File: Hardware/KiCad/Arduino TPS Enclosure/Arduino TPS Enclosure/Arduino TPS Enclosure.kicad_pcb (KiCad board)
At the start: 2 copper layers, 73.7 x 91.4 mm, 3 parts

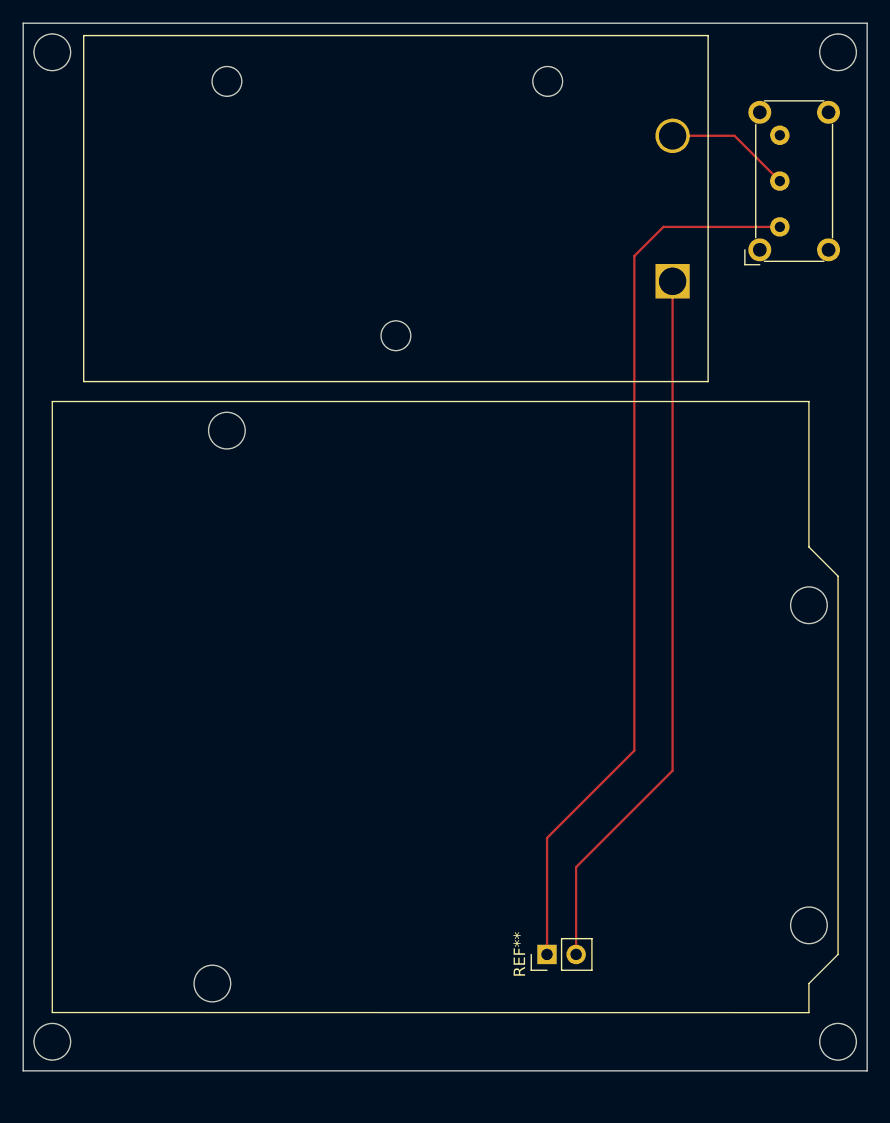
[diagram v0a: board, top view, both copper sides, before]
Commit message: Update
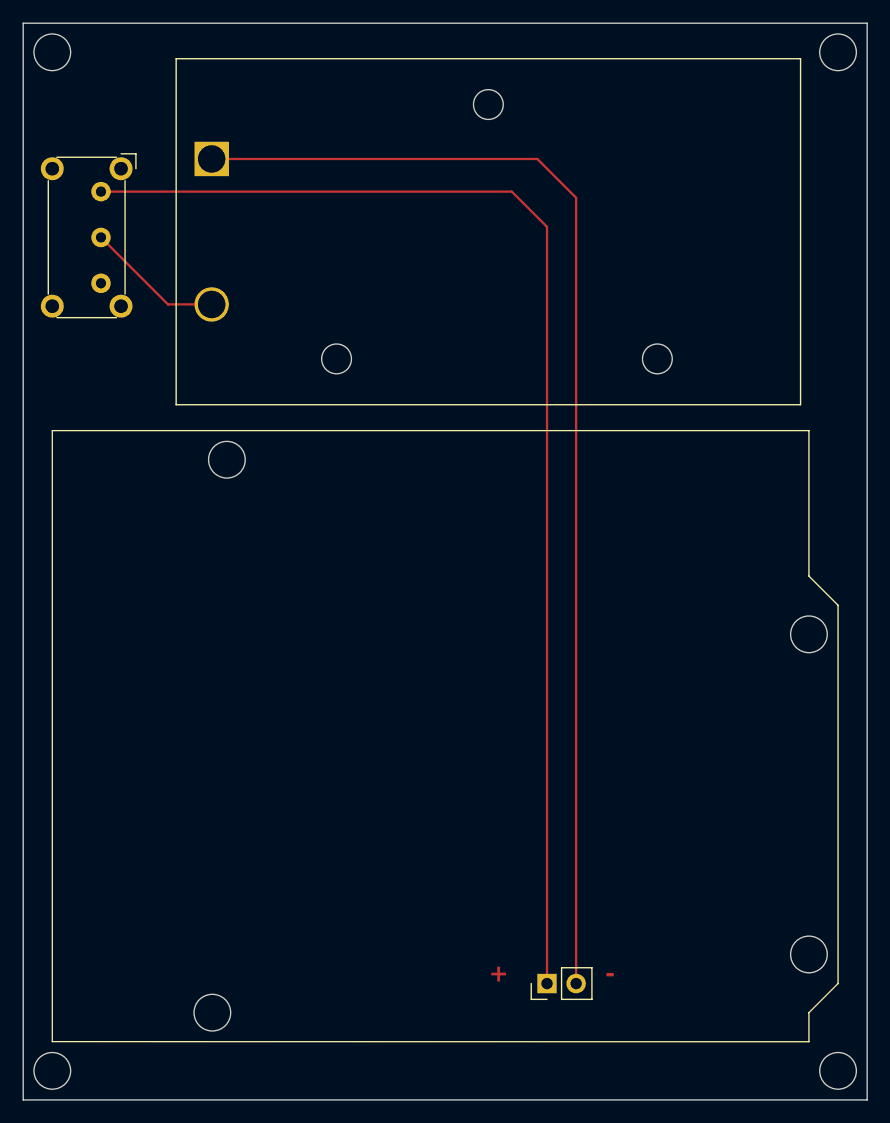
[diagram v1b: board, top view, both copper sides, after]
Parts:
- removed the REF** at (71.1, 106.7)
- added Vin: PinHeader_1x02_P2.54mm_Vertical, Connector_PinHeader_2.54mm:PinHeader_1x02_P2.54mm_Vertical, F.Cu at (71.1, 109.2)
- moved REF** 59.3 mm to (32.2, 40.1), turned to -90 degrees
- moved REF** 41.6 mm to (41.9, 37.2), turned to 180 degrees
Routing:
- net (no net): track 151.1 -> 220.1 mm
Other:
- board size 73.7 x 91.4 mm -> 73.7 x 94 mm
- board text added: "+"
- board text added: "-"
